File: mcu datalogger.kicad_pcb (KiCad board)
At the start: 2 copper layers, 50 x 30.5 mm, 29 parts, among them J1 Conn_01x04_Pin, J2 Conn_01x04_Pin, J3 Conn_01x09_Pin, J4 Conn_02x03_Odd_Even, U1 24LC1025, U2 24LC1025, U3 DS1337S_, U4 ATMEGA328P-AU, Y1 32.768KHz, Y2 16MHz

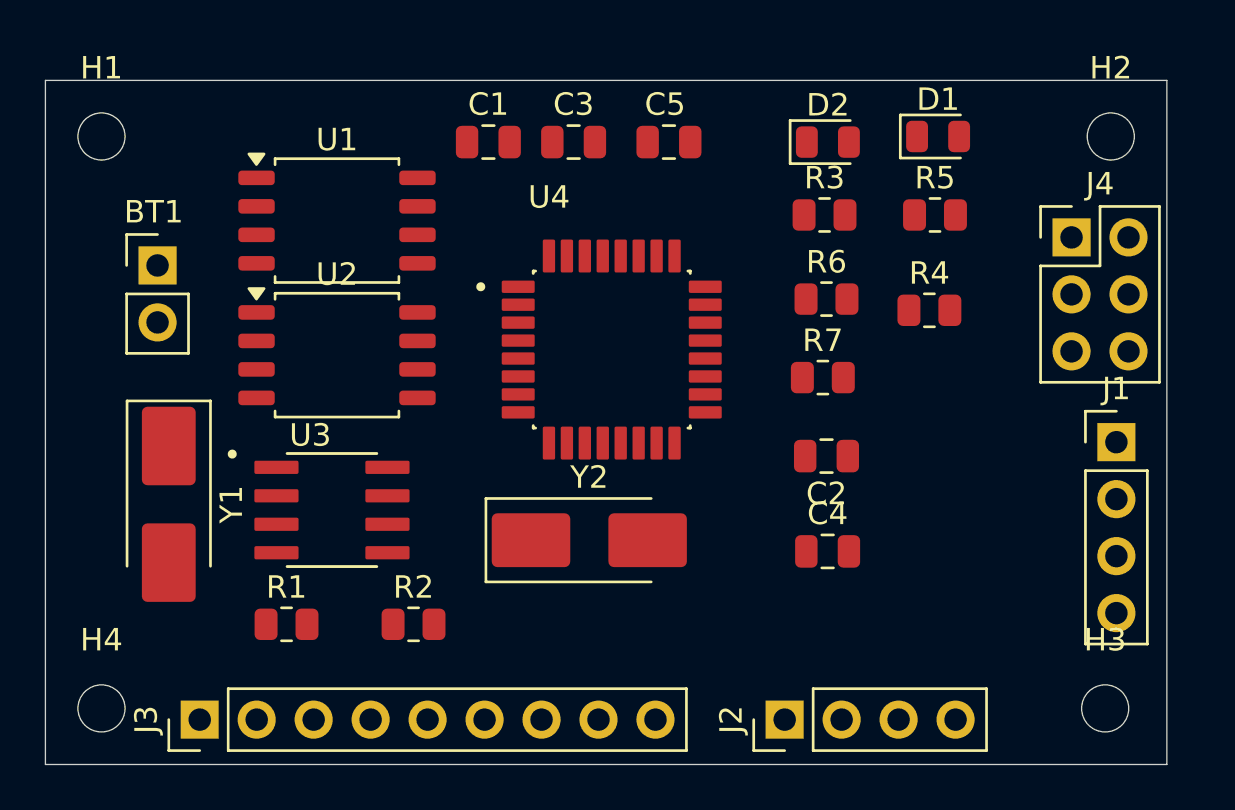
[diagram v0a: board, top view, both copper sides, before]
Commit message: Routing sans GND and Vcc completed
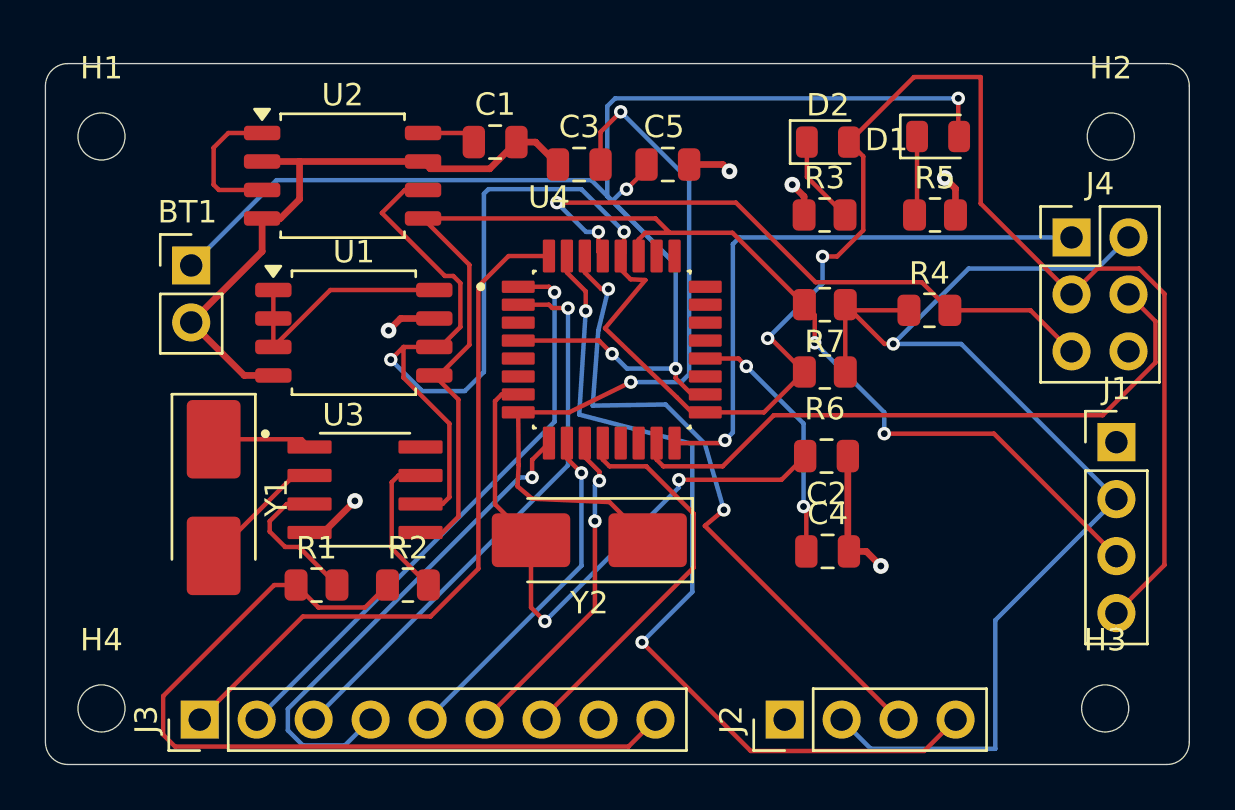
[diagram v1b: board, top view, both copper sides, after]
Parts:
- moved U2 8.00 mm to (165.8, 100.5)
- moved U1 5.06 mm to (166.2, 107.5)
- moved R7 3.25 mm to (187.2, 106.2), turned to 180 degrees
- moved R6 3.25 mm to (187.2, 109.2), turned to 180 degrees
- moved R1 2.20 mm to (164.6, 118.8)
- moved Y1 2.02 mm to (160.0, 114.8)
- moved R2 1.77 mm to (168.7, 118.8)
- moved U3 1.73 mm to (166.8, 114.5)
- moved BT1 1.50 mm to (159.0, 104.5)
- moved C3 1.03 mm to (176.3, 100.0)
- moved C5 1.00 mm to (180.2, 100.0)
- moved C1 0.30 mm to (172.6, 99.0)
- turned Y2 to 180 degrees
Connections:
- U1 pad 5: unconnected-(U1-SDA-Pad5) -> /SDA
- U2 pad 5: unconnected-(U2-SDA-Pad5) -> /SDA
- U3 pad 5: unconnected-(U3-SDA-Pad5) -> /SDA
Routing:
- net /Vcc: track 0.00 -> 111.6 mm, vias 0 -> 1
- net /SCK: track 0.00 -> 110.9 mm, vias 0 -> 4
- net Net-(BT1-+): track 0.00 -> 67.1 mm, vias 0 -> 4
- net /SDA: track 0.00 -> 58.0 mm, vias 0 -> 2
- net GND: track 0.00 -> 45.1 mm, vias 0 -> 6
- net /TX: track 0.00 -> 39.0 mm, vias 0 -> 2
- net Net-(U4-PB7): track 0.00 -> 33.8 mm, vias 0 -> 2
- net /D2: track 0.00 -> 31.5 mm
- net /RX: track 0.00 -> 29.5 mm, vias 0 -> 2
- net /RESET: track 0.00 -> 29.2 mm, vias 0 -> 2
- net /MOSI: track 0.00 -> 28.6 mm
- net Net-(U4-PB6): track 0.00 -> 26.9 mm, vias 0 -> 2
- net /MISO: track 0.00 -> 26.4 mm, vias 0 -> 1
- net /D3: track 0.00 -> 26.3 mm, vias 0 -> 1
- net /D4: track 0.00 -> 25.3 mm, vias 0 -> 1
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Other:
- board size 50 x 30.5 mm -> 51 x 31.2 mm
